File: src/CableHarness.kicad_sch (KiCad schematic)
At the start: 11 parts, among them J4 MiniFit_2x08_M

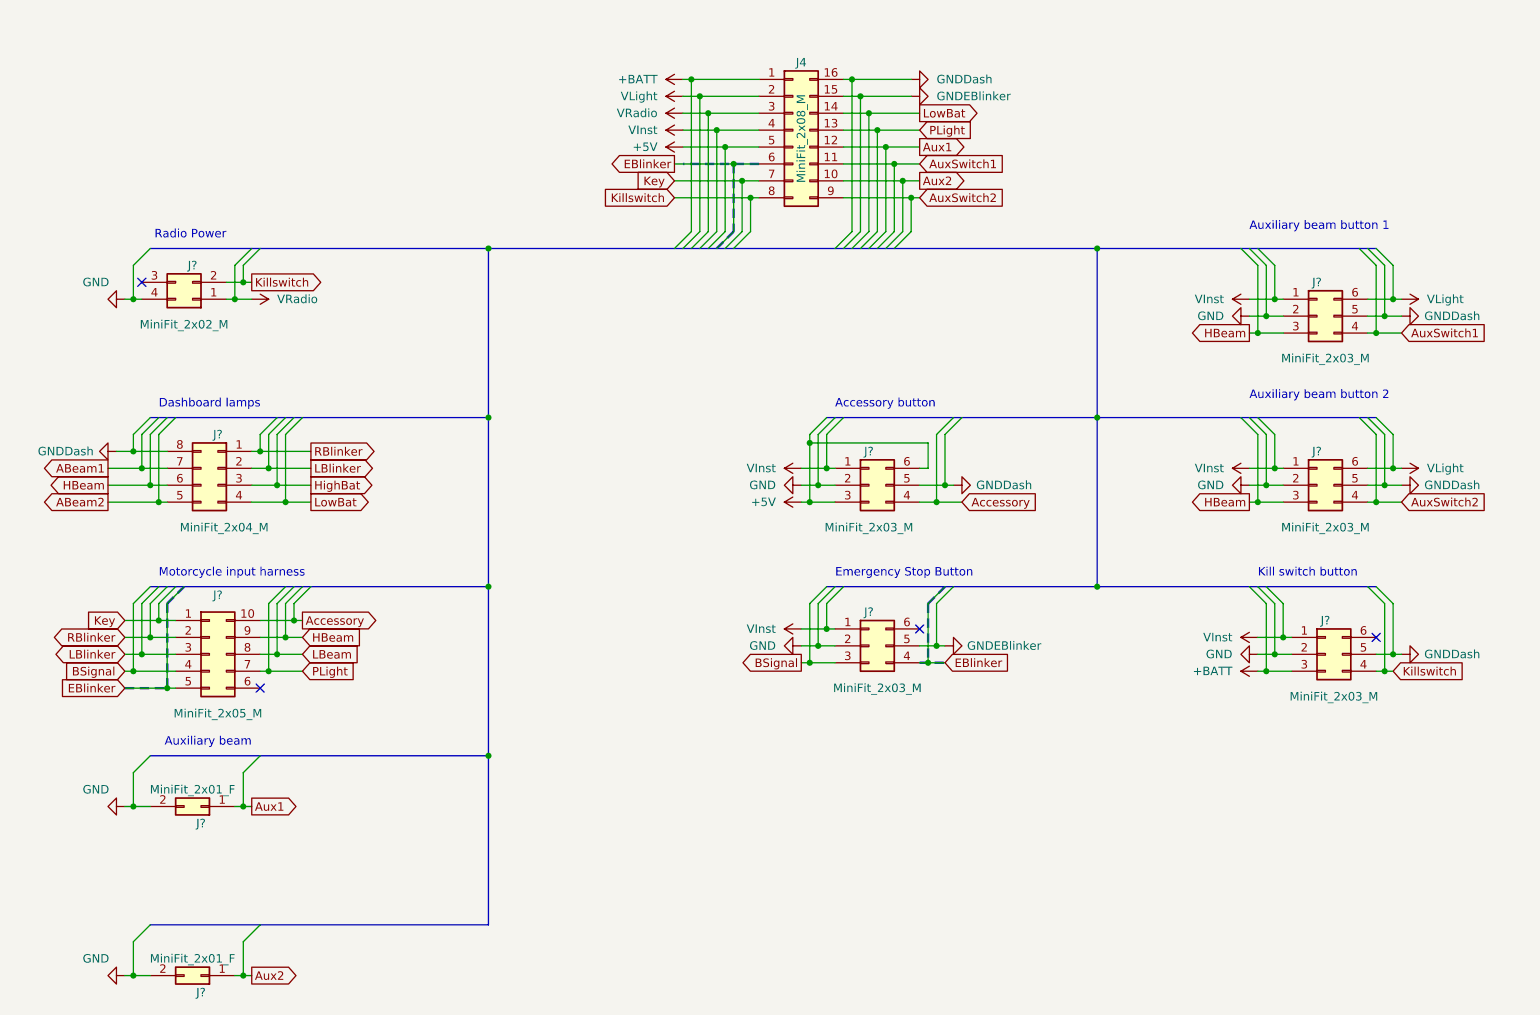
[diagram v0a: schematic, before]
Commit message: update Schematics
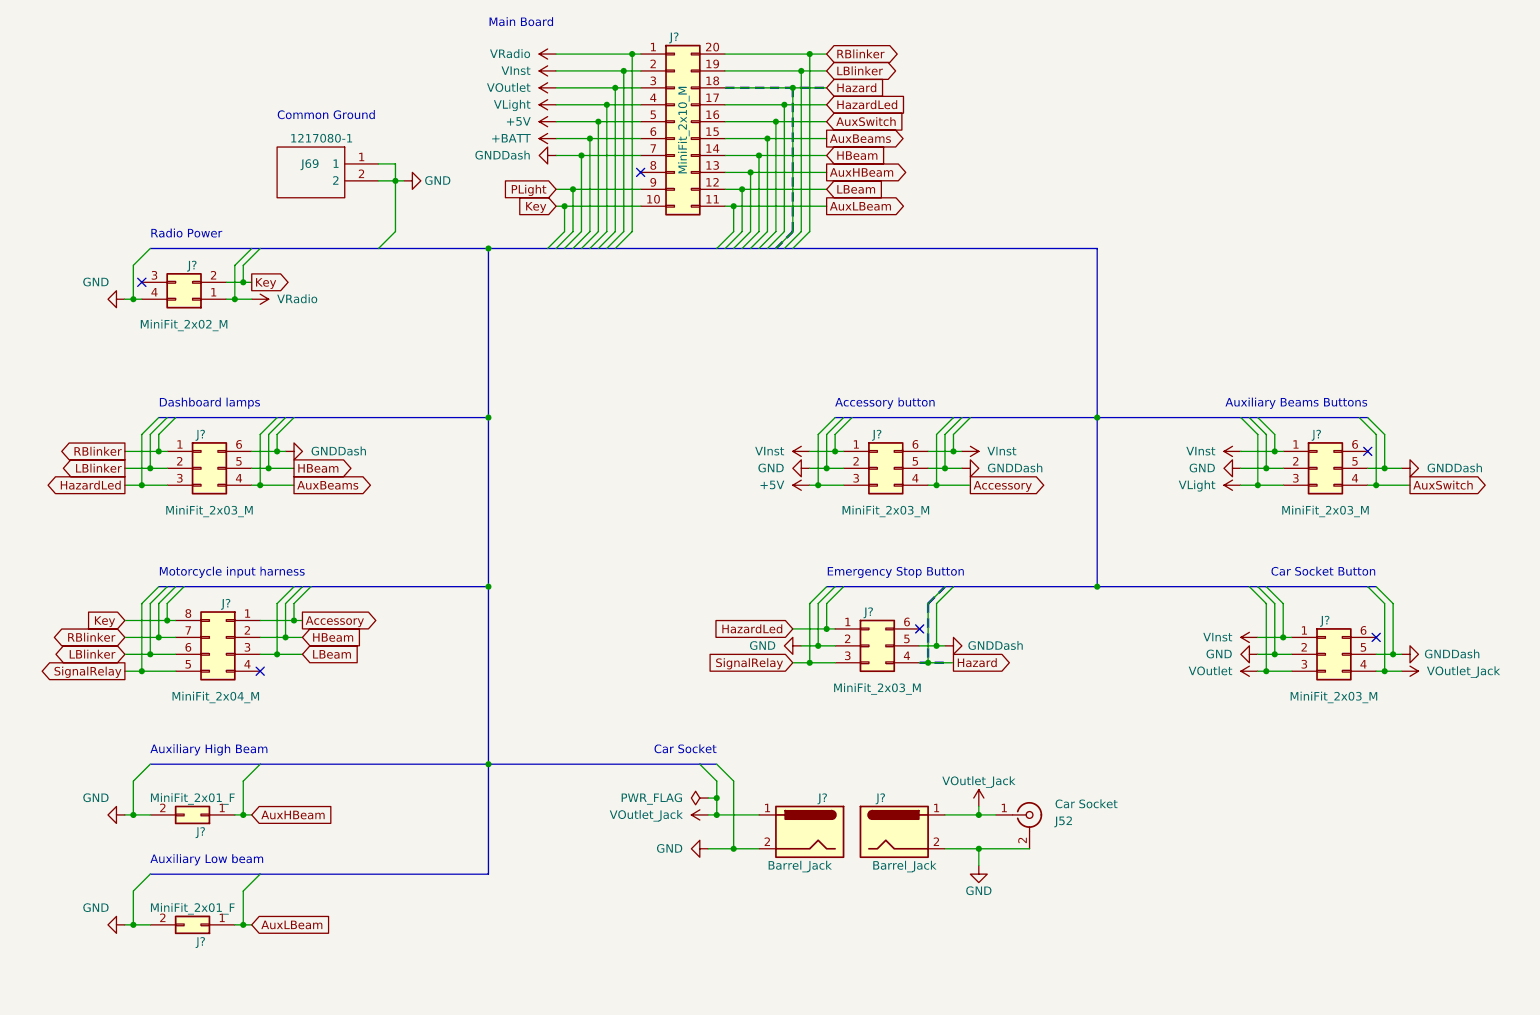
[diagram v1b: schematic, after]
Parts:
- removed J4: MiniFit_2x08_M, Connector_Molex:Molex_Mini-Fit_Jr_5566-16A_2x08_P4.20mm_Vertical, symbol Connector_Generic:Conn_02x08_Counter_Clockwise
- removed J? (x4): MiniFit_2x03_M, Connector_Molex:Molex_Mini-Fit_Jr_5566-06A_2x03_P4.20mm_Vertical, symbol Connector_Generic:Conn_02x03_Counter_Clockwise
- removed J?: MiniFit_2x01_F, Connector_Molex:Molex_Mini-Fit_Jr_5566-02A_2x01_P4.20mm_Vertical, symbol Connector_Generic:Conn_02x01
- removed J?: MiniFit_2x05_M, Connector_Molex:Molex_Mini-Fit_Jr_5566-10A_2x05_P4.20mm_Vertical, symbol Connector_Generic:Conn_02x05_Counter_Clockwise
- removed J?: MiniFit_2x04_M, Connector_Molex:Molex_Mini-Fit_Jr_5566-08A_2x04_P4.20mm_Vertical, symbol Connector_Generic:Conn_02x04_Counter_Clockwise
- added J52: Car Socket, symbol Connector:Conn_Coaxial
- added J69: 1217080-1, 1217080-1, symbol SamacSys_Parts:1217080-1
- added J?: MiniFit_2x10_M, symbol Connector_Generic:Conn_02x10_Counter_Clockwise
- added J?: MiniFit_2x04_M, Connector_Molex:Molex_Mini-Fit_Jr_5566-08A_2x04_P4.20mm_Vertical, symbol Connector_Generic:Conn_02x04_Counter_Clockwise
- added J? (x2): Barrel_Jack, Connector_BarrelJack:BarrelJack_CUI_PJ-063AH_Horizontal, symbol Connector:Barrel_Jack
- added J?: MiniFit_2x01_F, Connector_Molex:Molex_Mini-Fit_Jr_5566-02A_2x01_P4.20mm_Vertical, symbol Connector_Generic:Conn_02x01
- added J? (x4): MiniFit_2x03_M, Connector_Molex:Molex_Mini-Fit_Jr_5566-06A_2x03_P4.20mm_Vertical, symbol Connector_Generic:Conn_02x03_Counter_Clockwise
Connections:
- net GNDEBlinker is gone; now on net GNDDash: J?.5 (Pin_5)
- net Killswitch is gone; now on net Key: J?.2 (Pin_2)
- net +5V: now also J?.3 (Pin_3), J?.5 (Pin_5)
- net +BATT: now also J?.6 (Pin_6)
- net Accessory: now also J?.1 (Pin_1), J?.4 (Pin_4)
- net GND: now also J52.2 (Ext), J69.1, J69.2, J?.2, J?.2, J?.2 (Pin_2), J?.2 (Pin_2), J?.2 (Pin_2), J?.2 (Pin_2)
- net GNDDash: now also J?.5 (Pin_5), J?.5 (Pin_5), J?.5 (Pin_5), J?.6 (Pin_6), J?.7 (Pin_7)
- net HBeam: now also J?.14 (Pin_14), J?.2 (Pin_2), J?.5 (Pin_5)
- net Key: now also J?.10 (Pin_10), J?.8 (Pin_8)
- net LBeam: now also J?.12 (Pin_12), J?.3 (Pin_3)
- net LBlinker: now also J?.19 (Pin_19), J?.2 (Pin_2), J?.6 (Pin_6)
- net PLight: now also J?.9 (Pin_9)
- net RBlinker: now also J?.1 (Pin_1), J?.20 (Pin_20), J?.7 (Pin_7)
- net VInst: now also J?.1 (Pin_1), J?.1 (Pin_1), J?.1 (Pin_1), J?.2 (Pin_2), J?.6 (Pin_6); no longer J?.1 (Pin_1)
- net VLight: now also J?.3 (Pin_3), J?.4 (Pin_4)
- net VRadio: now also J?.1 (Pin_1)
- net Aux1 renamed AuxHBeam
- net AuxHBeam: now also J?.13 (Pin_13)
- net BSignal renamed SignalRelay
- net SignalRelay: now also J?.5 (Pin_5)
- net EBlinker renamed Hazard
- net Hazard: now also J?.18 (Pin_18)
- new net AuxBeams: J?.15 (Pin_15), J?.4 (Pin_4)
- new net AuxLBeam: J?.1 (Pin_1), J?.11 (Pin_11)
- new net AuxSwitch: J?.16 (Pin_16), J?.4 (Pin_4)
- new net HazardLed: J?.1 (Pin_1), J?.17 (Pin_17), J?.3 (Pin_3)
- new net VOutlet: J?.3 (Pin_3), J?.3 (Pin_3)
- new net VOutlet_Jack: J52.1 (In), J?.1, J?.1, J?.4 (Pin_4)
- no-connect marks 4 -> 6
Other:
- note added: "Auxiliary Beams Buttons"
- note added: "Auxiliary High Beam"
- note added: "Auxiliary Low beam"
- note added: "Car Socket"
- note added: "Car Socket Button"
- note added: "Common Ground"
- note added: "Main Board"
- note removed: "Auxiliary beam"
- note removed: "Auxiliary beam button 1"
- note removed: "Auxiliary beam button 2"
- note removed: "Kill switch button"
- moved on the sheet: J?
